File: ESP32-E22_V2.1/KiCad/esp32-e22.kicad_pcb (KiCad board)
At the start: 2 copper layers, 69.9 x 97.8 mm, 36 parts, among them J1 Conn_01x04_Socket, J10 Conn_01x02_Socket, J3 Conn_01x04_Socket, J4 Conn_01x03_Socket, J5 SMA, J6 Conn_01x02_Socket, J7 USB_C_Receptacle_PowerOnly_6P, J8 Conn_01x04_Socket, J9 Conn_01x02_Socket, SW1 SW_Push, U1 E22-40033S, U2 ESP32-DevKitC, U3 DM-OLED096-636

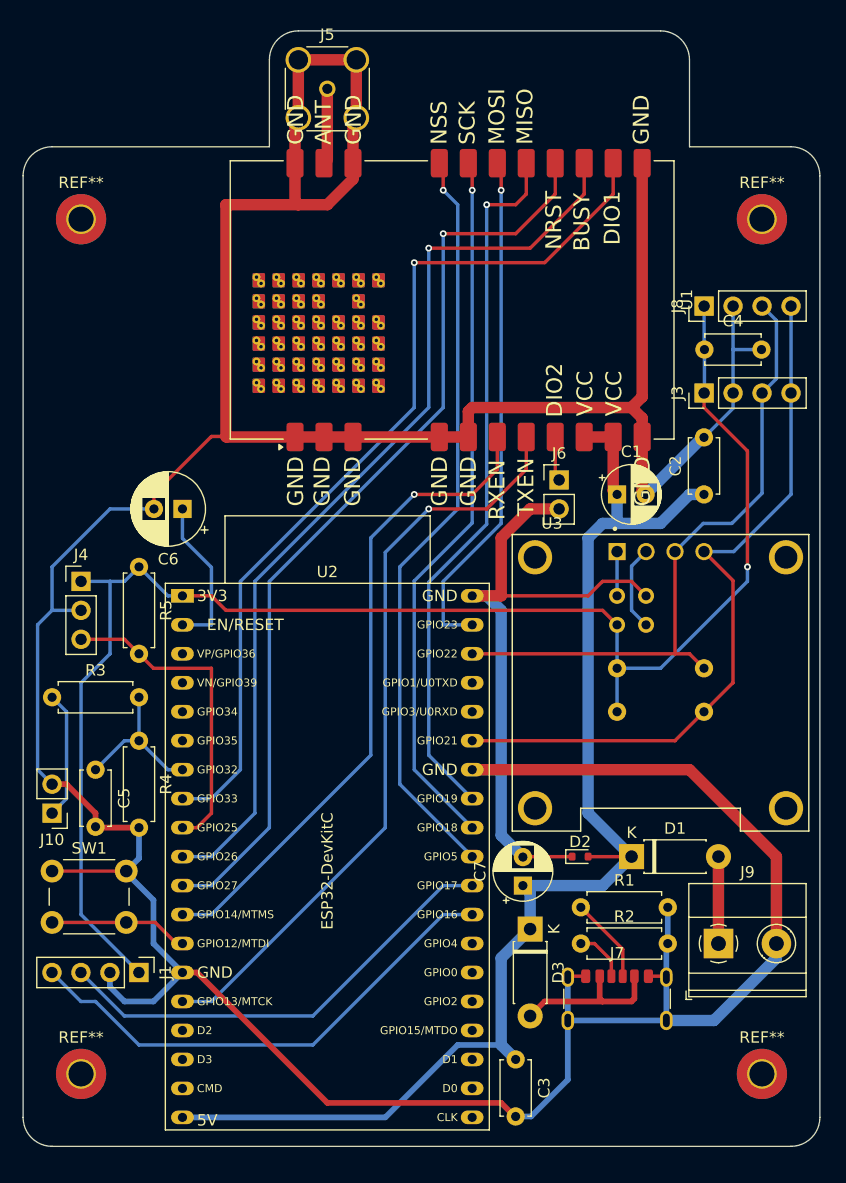
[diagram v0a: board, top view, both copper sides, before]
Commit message: new Version 2.0.10 & 2.0.6
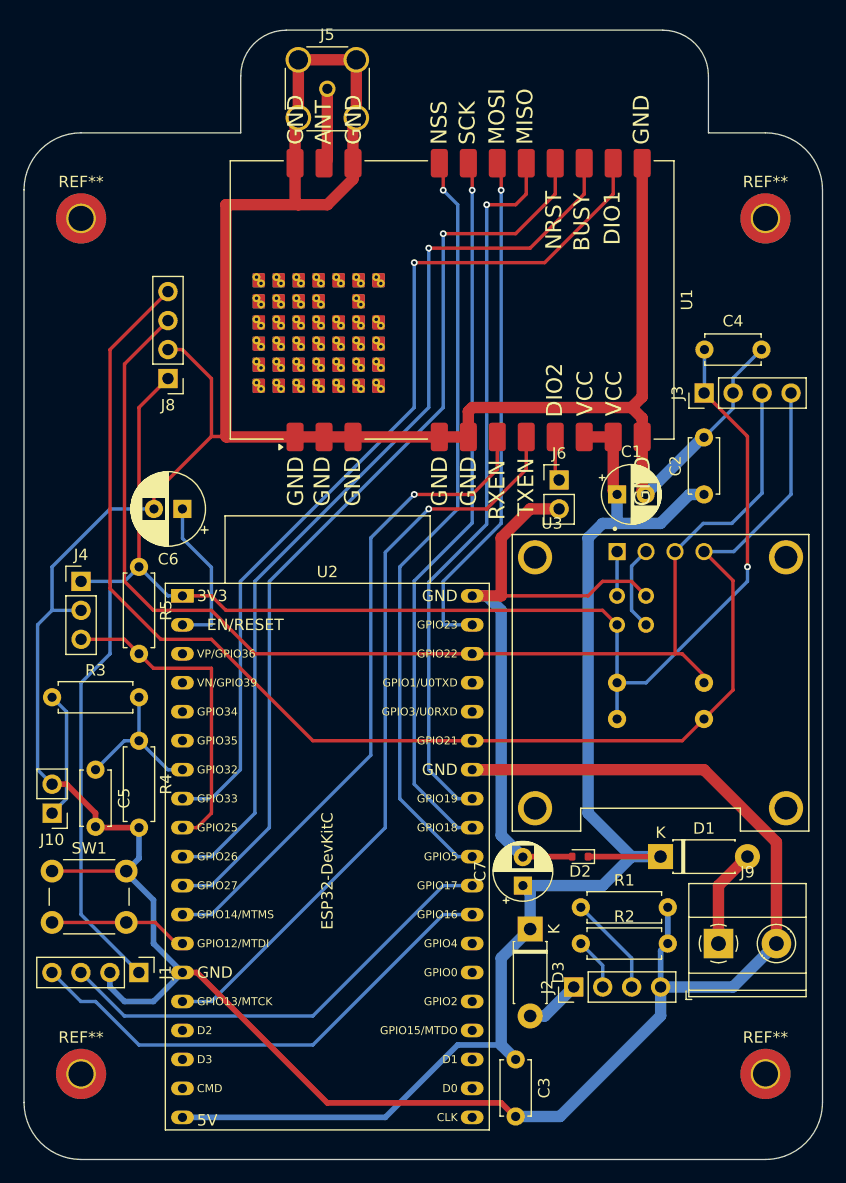
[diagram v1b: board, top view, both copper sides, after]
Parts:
- removed J7: USB_C_Receptacle_PowerOnly_6P, Connector_USB:USB_C_Receptacle_GCT_USB4125-xx-x-0190_6P_TopMnt_Horizontal
- added J2: Conn_01x04_Socket, Connector_PinHeader_2.54mm:PinHeader_1x04_P2.54mm_Vertical, F.Cu at (158.8, 130.8)
- moved J8 47.4 mm to (123.2, 77.5), turned to 180 degrees
- moved D1 2.54 mm to (166.4, 119.4)
- moved R7 1.27 mm to (162.6, 104.1)
- moved R6 0.63 mm to (162.6, 107.3)
- moved REF** 0.32 mm to (175.6, 63.4)
- moved REF** 0.31 mm to (175.6, 138.4)
- moved REF** 0.07 mm to (115.6, 63.4)
- turned D2 to 180 degrees
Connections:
- D2 pad 1: GND -> +5V
- D2 pad 2: +5V -> GND
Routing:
- net /SDA: track 63.7 -> 121.9 mm
- net /SCL: track 57.0 -> 106.2 mm
- net +3.3V: track 135.9 -> 150.8 mm
- net Net-(D3-A): track 14.1 -> 4.87 mm
- net GND: track 417.2 -> 410.3 mm
- net +5V: track 113.6 -> 118.6 mm
- net Net-(J2-Pin_3): track 7.56 -> 8.83 mm
- net Net-(D1-A): track 7.62 -> 8.67 mm
- net /MISO: track 62.3 -> 63.1 mm
- net /E22_SCK: track 62.6 -> 63.3 mm
- net /E22_NSS: track 66.2 -> 66.9 mm
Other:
- board size 69.9 x 97.8 mm -> 70 x 99 mm
